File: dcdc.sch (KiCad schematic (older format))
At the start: 9 parts, among them IC2 OKR-T_6-W12-C, J2 Conn_02x03_Counter_Clockwise

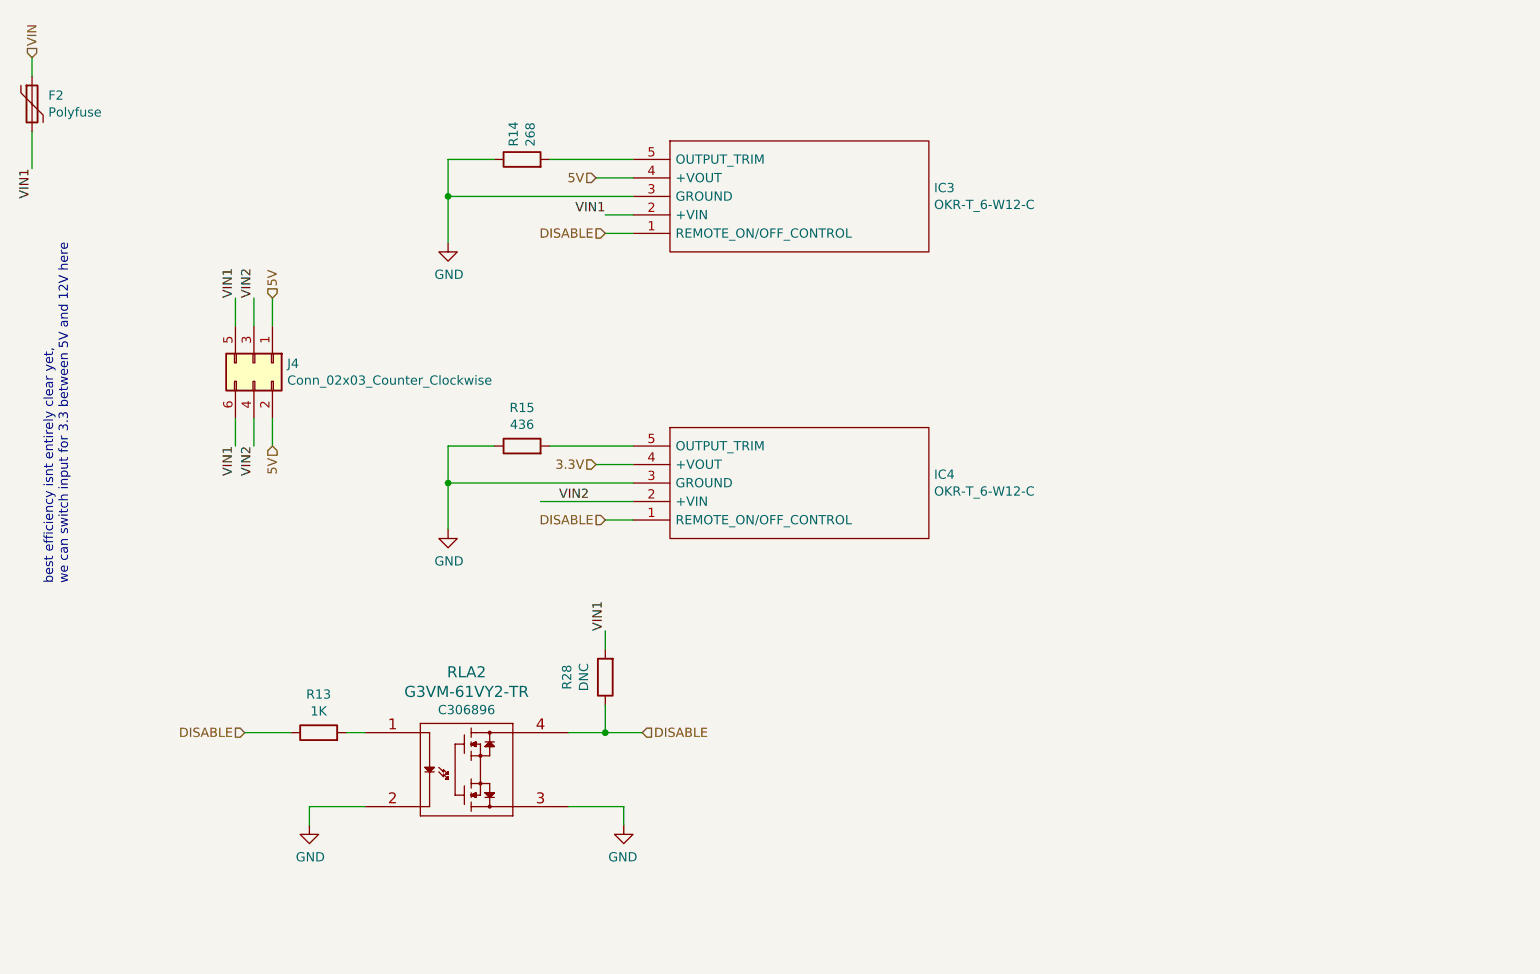
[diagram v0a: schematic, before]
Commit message: Organized DC-DC Schematic.
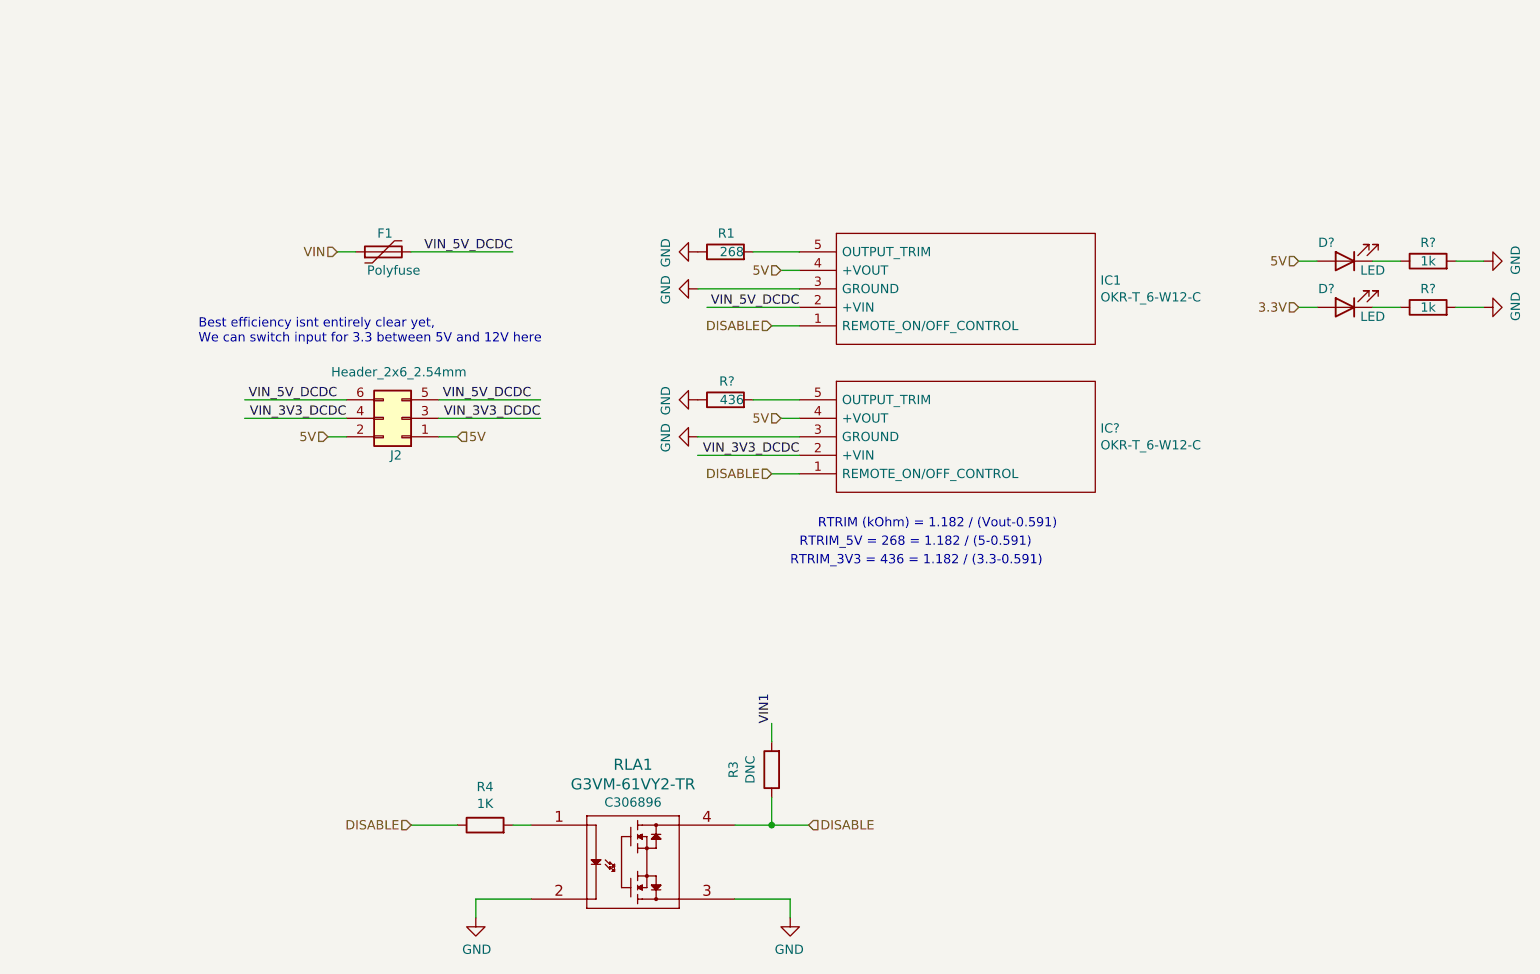
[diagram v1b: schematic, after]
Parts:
- removed IC2: OKR-T_6-W12-C, dg_power:MURATACASEC90, symbol dg_power:OKR-T_6-W12-C
- removed R2: 436, Resistor_SMD:R_0402_1005Metric_Pad0.72x0.64mm_HandSolder, symbol Device:R
- added D? (x2): LED, LED_SMD:LED_0603_1608Metric, symbol Device:LED
- added IC?: OKR-T_6-W12-C, dg_power:MURATACASEC90, symbol dg_power:OKR-T_6-W12-C
- added R? (x2): 1k, Resistor_SMD:R_0402_1005Metric, symbol Device:R
- added R?: 436, Resistor_SMD:R_0402_1005Metric_Pad0.72x0.64mm_HandSolder, symbol Device:R
- J2: value Conn_02x03_Counter_Clockwise -> Header_2x6_2.54mm
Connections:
- net labels added: VIN_3V3_DCDC, VIN_5V_DCDC
- net labels removed: VIN2
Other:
- note added: "Best efficiency isnt entirely clear yet,\nWe can switch input for 3.3 between 5V and 12V here"
- note added: "RTRIM (kOhm) = 1.182 / (Vout-0.591)"
- note added: "RTRIM_3V3 = 436 = 1.182 / (3.3-0.591)"
- note added: "RTRIM_5V = 268 = 1.182 / (5-0.591)"
- note removed: "best efficiency isnt entirely clear yet,\nwe can switch input for 3.3 between 5V and 12V here"
- moved on the sheet: F1, IC1, J2, R1, R3, R4, RLA1
